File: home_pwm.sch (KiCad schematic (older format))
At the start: 53 parts, among them J1 X977B06, J2 IDC-06, Q1 IRLR3410, Q2 IRLR3410, Q3 L-7113P3C, SW1 SW, SW2 SW, U1 ATmega8A-16AU, U2 L7805CDT, U3 IR25600, Y1 16 MHz

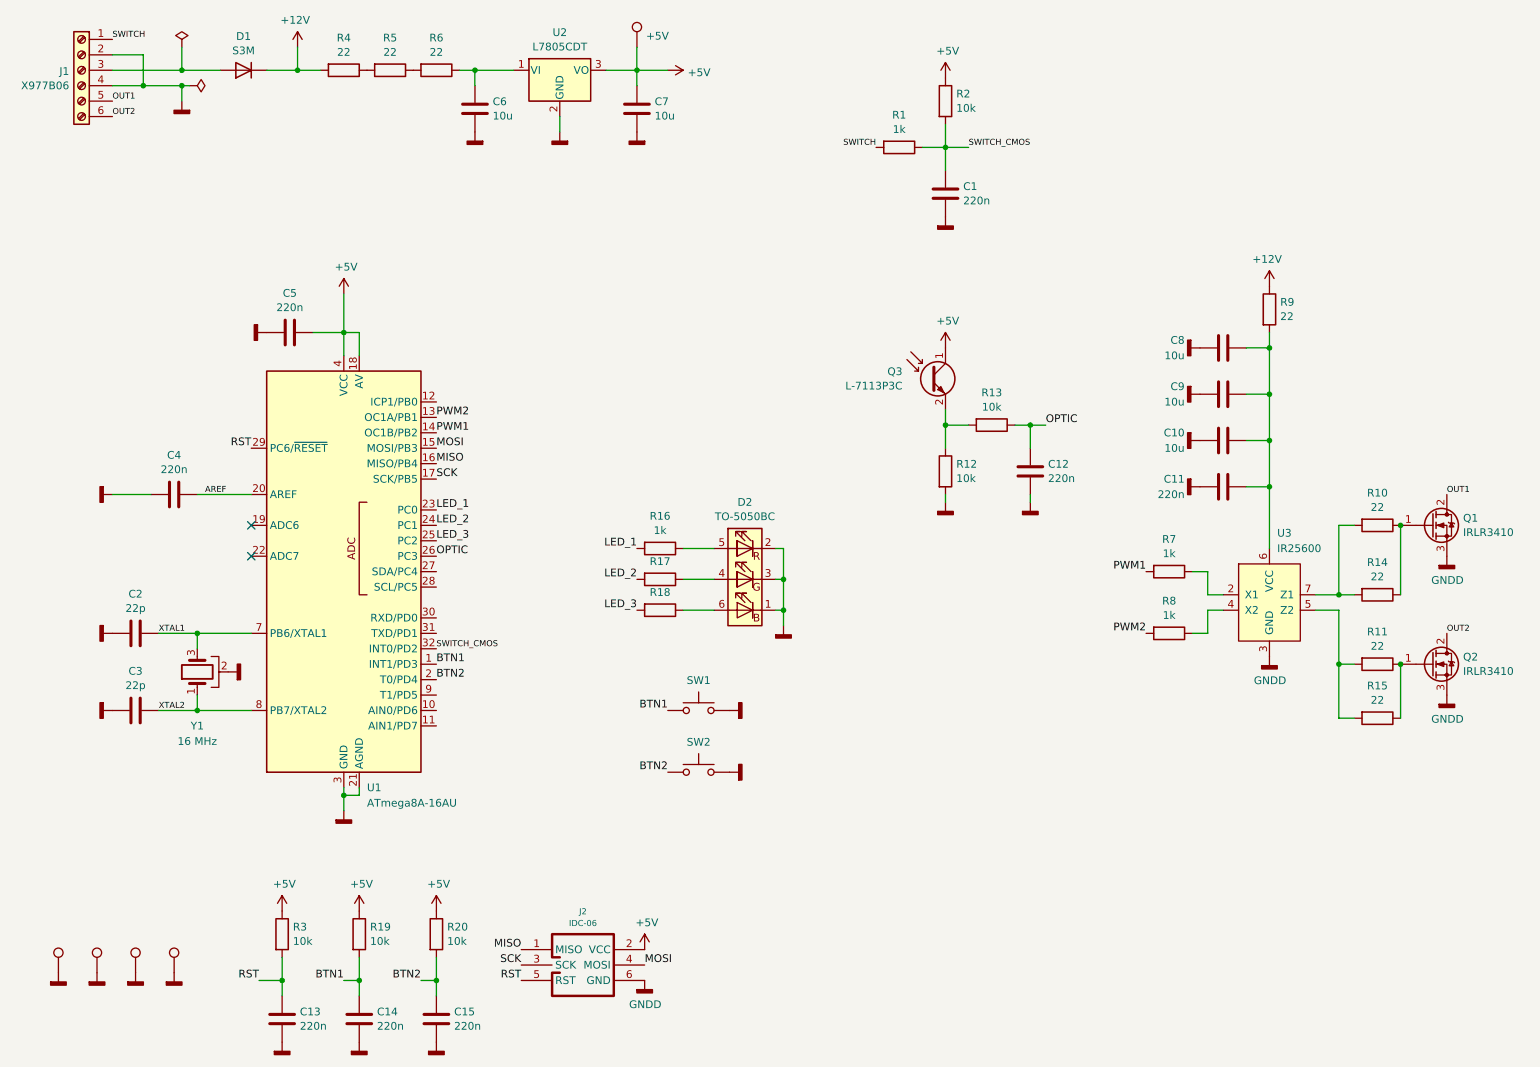
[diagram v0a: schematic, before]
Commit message: Gerbers
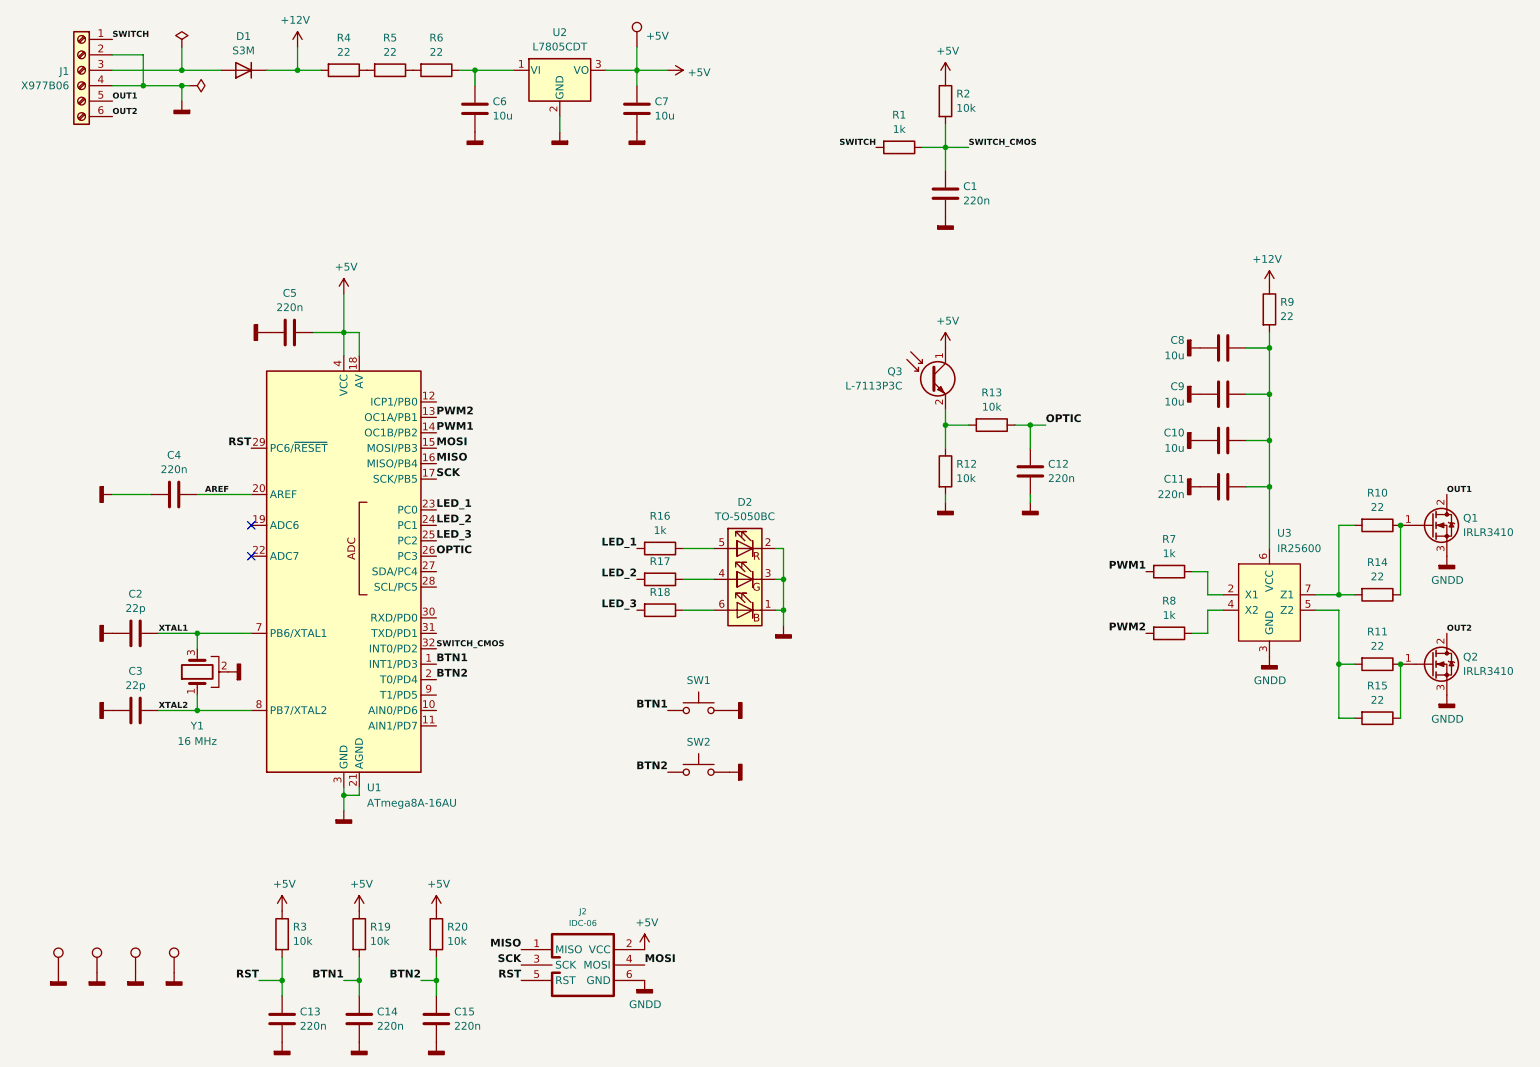
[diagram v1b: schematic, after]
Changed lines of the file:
@@
 	1    0    0    -1
 $EndComp
-Text Label 5450 7100 0    50   ~ 0
+Text Label 5450 7100 0    50   ~ 8
 MOSI
-Text Label 4650 7000 2    50   ~ 0
+Text Label 4650 7000 2    50   ~ 8
 MISO
-Text Label 4650 7100 2    50   ~ 0
+Text Label 4650 7100 2    50   ~ 8
 SCK
-Text Label 4650 7200 2    50   ~ 0
+Text Label 4650 7200 2    50   ~ 8
 RST
-Text Label 4100 3850 0    50   ~ 0
+Text Label 4100 3850 0    50   ~ 8
 MISO
-Text Label 4100 3950 0    50   ~ 0
+Text Label 4100 3950 0    50   ~ 8
 SCK
-Text Label 2900 3750 2    50   ~ 0
+Text Label 2900 3750 2    50   ~ 8
 RST
-Text Label 4100 3750 0    50   ~ 0
+Text Label 4100 3750 0    50   ~ 8
 MOSI
-Text Label 2950 7200 2    50   ~ 0
+Text Label 2950 7200 2    50   ~ 8
 RST
 $Comp
@@
 Wire Wire Line
 	3100 7200 3100 7050
-Text Label 4100 3650 0    50   ~ 0
+Text Label 4100 3650 0    50   ~ 8
 PWM1
-Text Label 4100 3550 0    50   ~ 0
+Text Label 4100 3550 0    50   ~ 8
 PWM2
-Text Label 8700 4550 2    50   ~ 0
+Text Label 8700 4550 2    50   ~ 8
 PWM1
-Text Label 8700 4950 2    50   ~ 0
+Text Label 8700 4950 2    50   ~ 8
 PWM2
 $Comp
@@
 	-1   0    0    -1
 $EndComp
-Text Label 2000 1500 0    39   ~ 0
+Text Label 2000 1500 0    39   ~ 7
 OUT1
-Text Label 2000 1600 0    39   ~ 0
+Text Label 2000 1600 0    39   ~ 7
 OUT2
 $Comp
@@
 	0    1    -1   0
 $EndComp
-Text Label 10650 4050 0    39   ~ 0
+Text Label 10650 4050 0    39   ~ 7
 OUT1
-Text Label 10650 4950 0    39   ~ 0
+Text Label 10650 4950 0    39   ~ 7
 OUT2
 $Comp
@@
 Wire Wire Line
 	2000 1400 2200 1400
-Text Label 2000 1100 0    39   ~ 0
+Text Label 2000 1100 0    39   ~ 7
 SWITCH
 Wire Wire Line
@@
 	7400 1650 7400 1800
 Connection ~ 7400 1800
-Text Label 6950 1800 2    39   ~ 0
+Text Label 6950 1800 2    39   ~ 7
 SWITCH
-Text Label 7550 1800 0    39   ~ 0
+Text Label 7550 1800 0    39   ~ 7
 SWITCH_CMOS
 Wire Wire Line
 	7550 1800 7400 1800
-Text Label 4100 5050 0    39   ~ 0
+Text Label 4100 5050 0    39   ~ 7
 SWITCH_CMOS
 NoConn ~ 2900 4250
@@
 	7950 3600 8050 3600
 Connection ~ 7950 3600
-Text Label 8050 3600 0    50   ~ 0
+Text Label 8050 3600 0    50   ~ 8
 OPTIC
-Text Label 4100 4450 0    50   ~ 0
+Text Label 4100 4450 0    50   ~ 8
 OPTIC
 $Comp
@@
 	1    0    0    -1
 $EndComp
-Text Label 2300 4950 0    39   ~ 0
+Text Label 2300 4950 0    39   ~ 7
 XTAL1
-Text Label 2300 5450 0    39   ~ 0
+Text Label 2300 5450 0    39   ~ 7
 XTAL2
-Text Label 2600 4050 0    39   ~ 0
+Text Label 2600 4050 0    39   ~ 7
 AREF
 $Comp
@@
 	9950 5500 9950 5150
 Connection ~ 9950 5150
-Text Label 4100 4150 0    50   ~ 0
+Text Label 4100 4150 0    50   ~ 8
 LED_1
-Text Label 4100 4250 0    50   ~ 0
+Text Label 4100 4250 0    50   ~ 8
 LED_2
-Text Label 4100 4350 0    50   ~ 0
+Text Label 4100 4350 0    50   ~ 8
 LED_3
-Text Label 5400 4400 2    50   ~ 0
+Text Label 5400 4400 2    50   ~ 8
 LED_1
-Text Label 5400 4600 2    50   ~ 0
+Text Label 5400 4600 2    50   ~ 8
 LED_2
-Text Label 5400 4800 2    50   ~ 0
+Text Label 5400 4800 2    50   ~ 8
 LED_3
 $Comp
@@
 	0    -1   -1   0
 $EndComp
-Text Label 5600 5450 2    50   ~ 0
+Text Label 5600 5450 2    50   ~ 8
 BTN1
-Text Label 5600 5850 2    50   ~ 0
+Text Label 5600 5850 2    50   ~ 8
 BTN2
-Text Label 4100 5150 0    50   ~ 0
+Text Label 4100 5150 0    50   ~ 8
 BTN1
-Text Label 4100 5250 0    50   ~ 0
+Text Label 4100 5250 0    50   ~ 8
 BTN2
 $Comp
@@
 	1    0    0    -1
 $EndComp
-Text Label 4000 7200 2    50   ~ 0
+Text Label 4000 7200 2    50   ~ 8
 BTN2
-Text Label 3500 7200 2    50   ~ 0
+Text Label 3500 7200 2    50   ~ 8
 BTN1
 $Comp
